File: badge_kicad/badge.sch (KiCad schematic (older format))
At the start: 22 parts, among them P1 Pin, P2 Pin, P3 Pin, P4 Pin, P5 Pin, P6 Pin, Q1 2N2222, SW1 ON

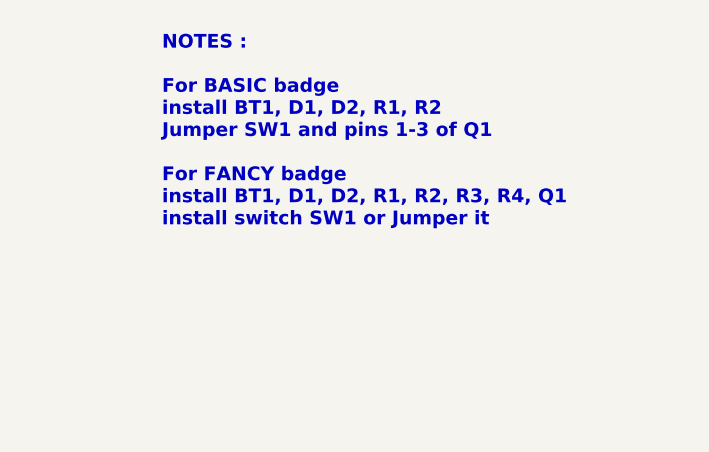
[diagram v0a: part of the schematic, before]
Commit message: schematic notes
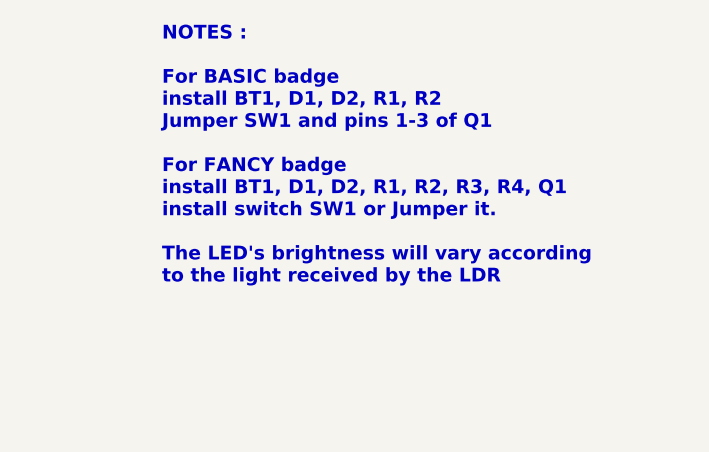
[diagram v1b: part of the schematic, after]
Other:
- note added: "NOTES :\n\nFor BASIC badge\ninstall BT1, D1, D2, R1, R2\nJumper SW1 and pins 1-3 of Q1\n\nFor FANCY badge\ninstall BT1, D1, D2, R1, R2, R3, R4, Q1\ninstall switch SW1 or Jumper it.\n\nThe LED's brightness will vary according\nto the light received by the LDR"
- note removed: "NOTES :\n\nFor BASIC badge\ninstall BT1, D1, D2, R1, R2\nJumper SW1 and pins 1-3 of Q1\n\nFor FANCY badge\ninstall BT1, D1, D2, R1, R2, R3, R4, Q1\ninstall switch SW1 or Jumper it"
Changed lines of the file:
@@
 	1    0    0    -1
 $EndComp
-Text Notes 9000 1550 0    60   ~ 12
-NOTES :\n\nFor BASIC badge\ninstall BT1, D1, D2, R1, R2\nJumper SW1 and pins 1-3 of Q1\n\nFor FANCY badge\ninstall BT1, D1, D2, R1, R2, R3, R4, Q1\ninstall switch SW1 or Jumper it
+Text Notes 9000 1800 0    60   ~ 12
+NOTES :\n\nFor BASIC badge\ninstall BT1, D1, D2, R1, R2\nJumper SW1 and pins 1-3 of Q1\n\nFor FANCY badge\ninstall BT1, D1, D2, R1, R2, R3, R4, Q1\ninstall switch SW1 or Jumper it.\n\nThe LED's brightness will vary according\nto the light received by the LDR
 Text Label 6000 4525 0    60   ~ 12
 Base
